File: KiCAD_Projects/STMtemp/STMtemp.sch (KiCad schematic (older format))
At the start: 11 parts, among them SW1 SW_PUSH, U1 STM32F103_48, X1 CRYSTAL, X2 CRYSTAL

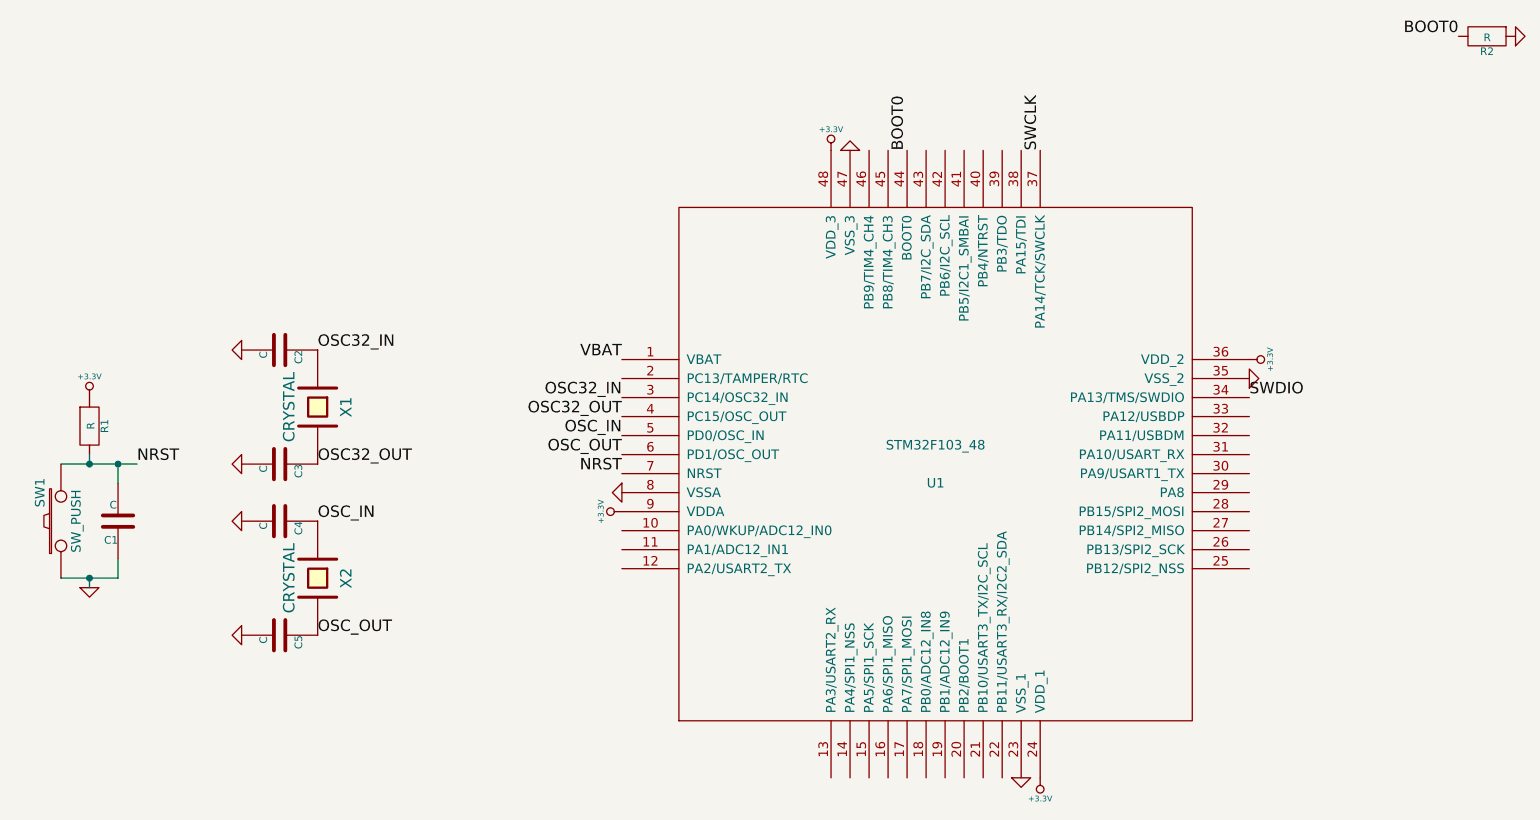
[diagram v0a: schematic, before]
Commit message: no message
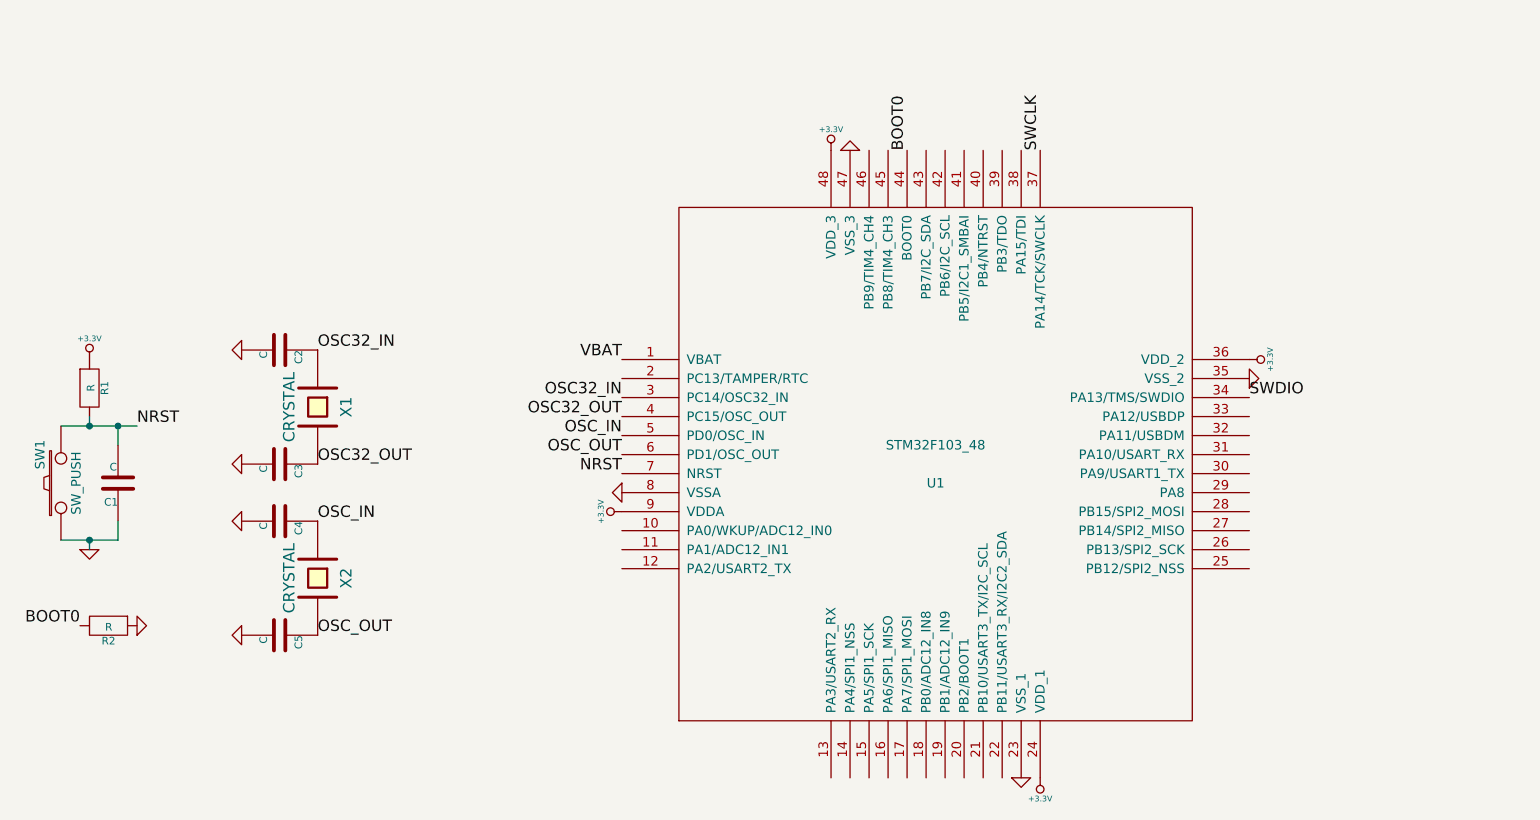
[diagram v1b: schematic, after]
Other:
- moved on the sheet: C1, R1, R2, SW1
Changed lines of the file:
@@
 LIBS:user
 LIBS:power
+LIBS:STMtemp-cache
 EELAYER 25 0
 EELAYER END
@@
 L SW_PUSH SW1
 U 1 1 5773C76A
-P 1050 4000
-F 0 "SW1" H 1200 4110 50  0000 C CNN
-F 1 "SW_PUSH" H 1050 3920 50  0000 C CNN
-F 2 "" H 1050 4000 60  0000 C CNN
-F 3 "" H 1050 4000 60  0000 C CNN
-	1    1050 4000
+P 1050 3800
+F 0 "SW1" H 1200 3910 50  0000 C CNN
+F 1 "SW_PUSH" H 1050 3720 50  0000 C CNN
+F 2 "" H 1050 3800 60  0000 C CNN
+F 3 "" H 1050 3800 60  0000 C CNN
+	1    1050 3800
 	0    -1   -1   0
 $EndComp
@@
 L C C1
 U 1 1 5773C845
-P 1350 4000
-F 0 "C1" H 1350 4100 40  0000 L CNN
-F 1 "C" H 1356 3915 40  0000 L CNN
-F 2 "" H 1388 3850 30  0000 C CNN
-F 3 "" H 1350 4000 60  0000 C CNN
-	1    1350 4000
+P 1350 3800
+F 0 "C1" H 1350 3900 40  0000 L CNN
+F 1 "C" H 1356 3715 40  0000 L CNN
+F 2 "" H 1388 3650 30  0000 C CNN
+F 3 "" H 1350 3800 60  0000 C CNN
+	1    1350 3800
 	-1   0    0    1
 $EndComp
@@
 L GND #PWR05
 U 1 1 5773CA03
-P 1200 4350
-F 0 "#PWR05" H 1200 4350 30  0001 C CNN
-F 1 "GND" H 1200 4280 30  0001 C CNN
-F 2 "" H 1200 4350 60  0000 C CNN
-F 3 "" H 1200 4350 60  0000 C CNN
-	1    1200 4350
-	1    0    0    -1
-$EndComp
-Wire Wire Line
-	1050 4300 1350 4300
-Wire Wire Line
-	1350 4300 1350 4200
-Wire Wire Line
-	1200 4300 1200 4350
-Connection ~ 1200 4300
-Wire Wire Line
-	1050 3700 1450 3700
-Wire Wire Line
-	1350 3700 1350 3800
+P 1200 4150
+F 0 "#PWR05" H 1200 4150 30  0001 C CNN
+F 1 "GND" H 1200 4080 30  0001 C CNN
+F 2 "" H 1200 4150 60  0000 C CNN
+F 3 "" H 1200 4150 60  0000 C CNN
+	1    1200 4150
+	1    0    0    -1
+$EndComp
+Wire Wire Line
+	1050 4100 1350 4100
+Wire Wire Line
+	1350 4100 1350 4000
+Wire Wire Line
+	1200 4100 1200 4150
+Connection ~ 1200 4100
+Wire Wire Line
+	1050 3500 1450 3500
+Wire Wire Line
+	1350 3500 1350 3600
 $Comp
 L R R1
 U 1 1 5773CB7C
-P 1200 3500
-F 0 "R1" V 1280 3500 40  0000 C CNN
-F 1 "R" V 1207 3501 40  0000 C CNN
-F 2 "" V 1130 3500 30  0000 C CNN
-F 3 "" H 1200 3500 30  0000 C CNN
-	1    1200 3500
-	1    0    0    -1
-$EndComp
-Wire Wire Line
-	1200 3650 1200 3700
-Connection ~ 1200 3700
+P 1200 3300
+F 0 "R1" V 1280 3300 40  0000 C CNN
+F 1 "R" V 1207 3301 40  0000 C CNN
+F 2 "" V 1130 3300 30  0000 C CNN
+F 3 "" H 1200 3300 30  0000 C CNN
+	1    1200 3300
+	1    0    0    -1
+$EndComp
+Wire Wire Line
+	1200 3450 1200 3500
+Connection ~ 1200 3500
 $Comp
 L +3.3V #PWR06
 U 1 1 5773CCAC
-P 1200 3350
-F 0 "#PWR06" H 1200 3310 30  0001 C CNN
-F 1 "+3.3V" H 1200 3460 30  0000 C CNN
-F 2 "" H 1200 3350 60  0000 C CNN
-F 3 "" H 1200 3350 60  0000 C CNN
-	1    1200 3350
-	1    0    0    -1
-$EndComp
-Connection ~ 1350 3700
-Text Label 1450 3700 0    60   ~ 0
+P 1200 3150
+F 0 "#PWR06" H 1200 3110 30  0001 C CNN
+F 1 "+3.3V" H 1200 3260 30  0000 C CNN
+F 2 "" H 1200 3150 60  0000 C CNN
+F 3 "" H 1200 3150 60  0000 C CNN
+	1    1200 3150
+	1    0    0    -1
+$EndComp
+Connection ~ 1350 3500
+Text Label 1450 3500 0    60   ~ 0
 NRST
 Text Label 4000 3750 2    60   ~ 0
@@
 L R R2
 U 1 1 5773D19C
-P 8550 1450
-F 0 "R2" V 8630 1450 40  0000 C CNN
-F 1 "R" V 8557 1451 40  0000 C CNN
-F 2 "" V 8480 1450 30  0000 C CNN
-F 3 "" H 8550 1450 30  0000 C CNN
-	1    8550 1450
+P 1300 4550
+F 0 "R2" V 1380 4550 40  0000 C CNN
+F 1 "R" V 1307 4551 40  0000 C CNN
+F 2 "" V 1230 4550 30  0000 C CNN
+F 3 "" H 1300 4550 30  0000 C CNN
+	1    1300 4550
 	0    1    1    0
 $EndComp
@@
 L GND #PWR07
 U 1 1 5773D3FC
-P 8700 1450
-F 0 "#PWR07" H 8700 1450 30  0001 C CNN
-F 1 "GND" H 8700 1380 30  0001 C CNN
-F 2 "" H 8700 1450 60  0000 C CNN
-F 3 "" H 8700 1450 60  0000 C CNN
-	1    8700 1450
+P 1450 4550
+F 0 "#PWR07" H 1450 4550 30  0001 C CNN
+F 1 "GND" H 1450 4480 30  0001 C CNN
+F 2 "" H 1450 4550 60  0000 C CNN
+F 3 "" H 1450 4550 60  0000 C CNN
+	1    1450 4550
 	0    -1   -1   0
 $EndComp
-Text Label 8400 1450 2    60   ~ 0
+Text Label 1150 4550 2    60   ~ 0
 BOOT0
 Text Label 5500 2050 1    60   ~ 0
